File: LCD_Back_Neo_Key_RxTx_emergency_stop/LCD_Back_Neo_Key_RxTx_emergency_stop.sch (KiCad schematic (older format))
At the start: 4 parts, among them J3 Conn_01x08_Male_KeyPad, U1 DC-DC_Stepdown-Zimprich

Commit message: update
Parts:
- A1: symbol MCU_Module:Arduino_Nano_v3.x -> LCD_Back_Neo_Key_RxTx_emergency_stop-rescue:Arduino_Nano_v3.x-MCU_Module
- J3: symbol Connector:Conn_01x08_Male -> LCD_Back_Neo_Key_RxTx_emergency_stop-rescue:Conn_01x08_Male-Connector
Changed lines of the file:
@@
 $EndDescr
 $Comp
-L MCU_Module:Arduino_Nano_v3.x A1
+L LCD_Back_Neo_Key_RxTx_emergency_stop-rescue:Arduino_Nano_v3.x-MCU_Module A1
 U 1 1 5CDFD485
 P 5400 4650
@@
 Ardu_A2
 $Comp
-L Connector:Conn_01x08_Male J3
+L LCD_Back_Neo_Key_RxTx_emergency_stop-rescue:Conn_01x08_Male-Connector J3
 U 1 1 5CE28136
 P 1400 6500

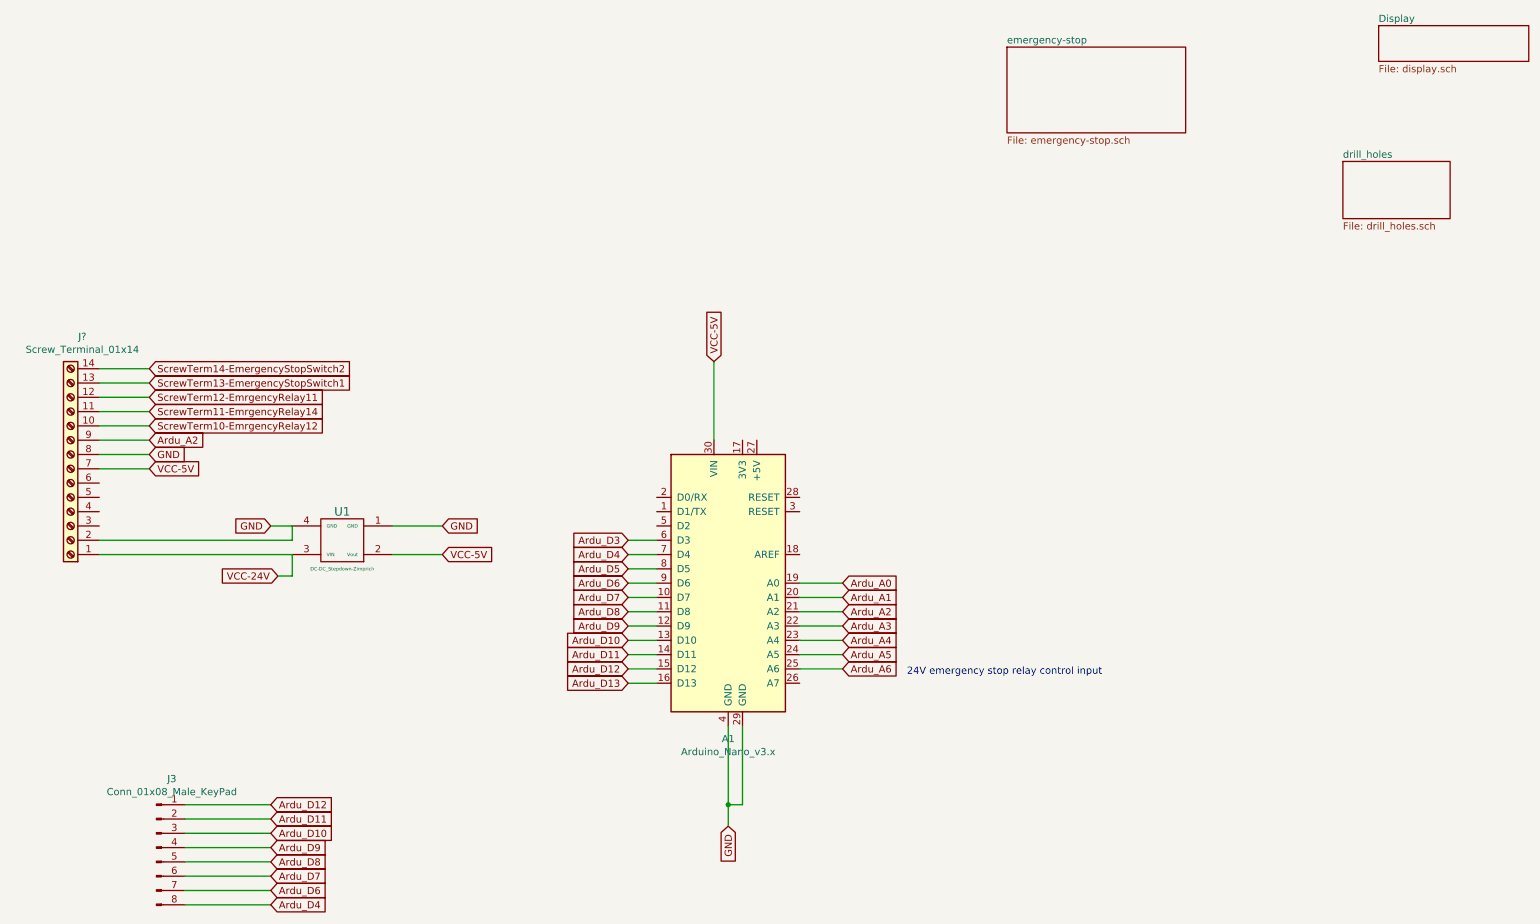
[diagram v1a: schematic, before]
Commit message: place screwterminal on PCB
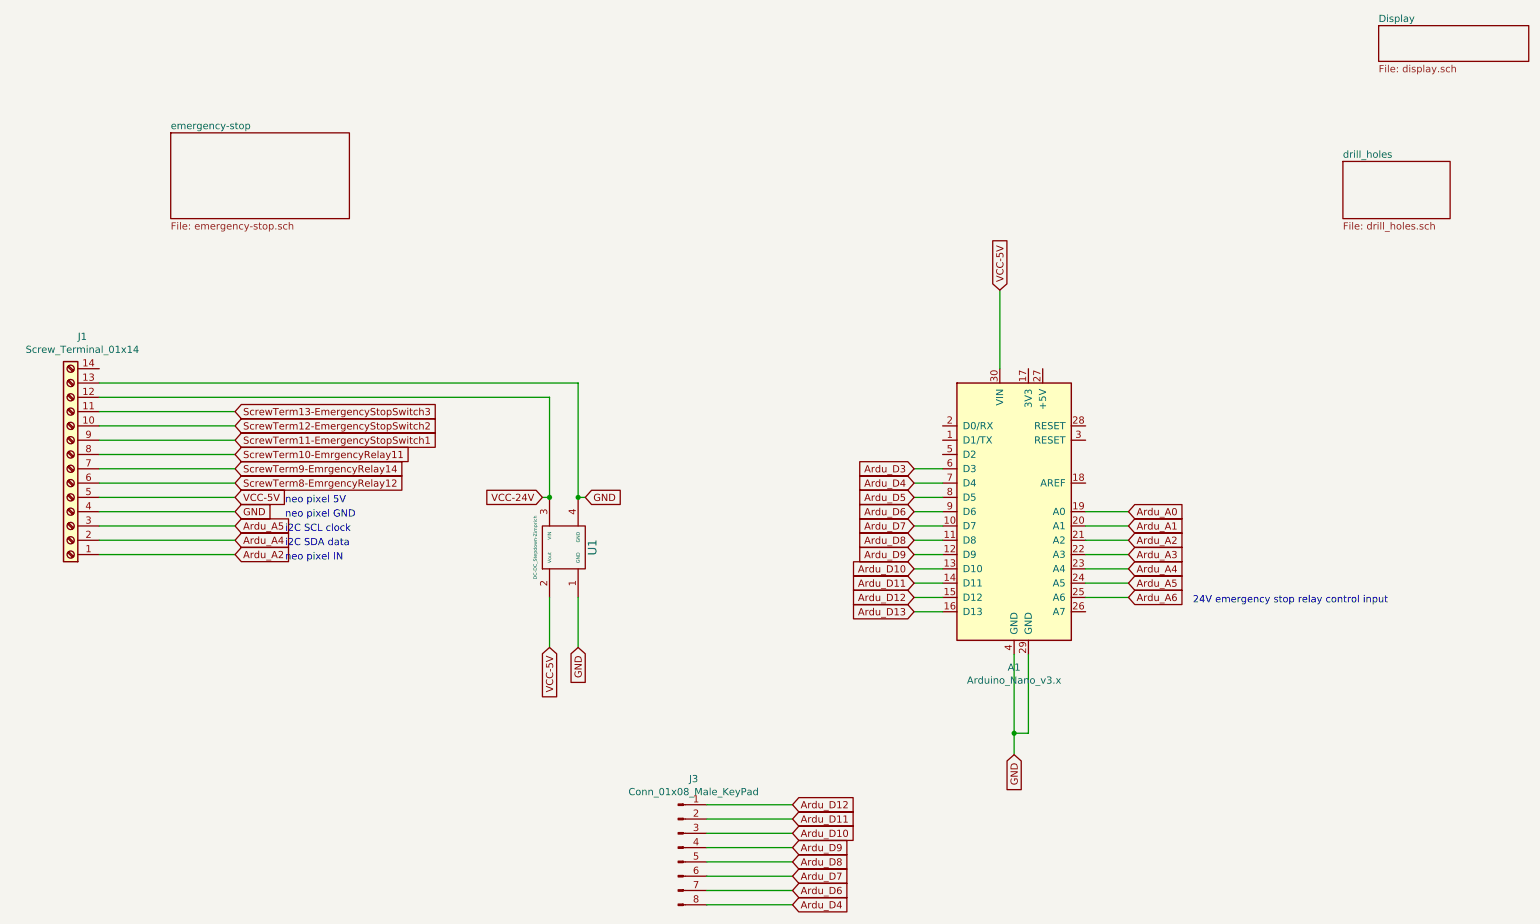
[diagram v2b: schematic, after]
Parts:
- J1: renamed from J?; footprint (none) -> Connector_Phoenix_MSTB:PhoenixContact_MSTBVA_2,5_14-G_1x14_P5.00mm_Vertical
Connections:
- net ScrewTerm12-EmrgencyRelay11 is gone; now on net VCC-24V: J1.12 (Pin_12)
- net ScrewTerm13-EmergencyStopSwitch1 is gone; now on net GND: J1.13 (Pin_13)
- net Ardu_A2: now also J1.1 (Pin_1); no longer J1.9 (Pin_9)
- net Ardu_A4: now also J1.2 (Pin_2)
- net Ardu_A5: now also J1.3 (Pin_3)
- net GND: now also J1.4 (Pin_4); no longer J1.2 (Pin_2), J1.8 (Pin_8)
- net VCC-24V: no longer J1.1 (Pin_1)
- net VCC-5V: now also J1.5 (Pin_5); no longer J1.7 (Pin_7)
- net ScrewTerm8-EmrgencyRelay12: now reaches J1.6 (Pin_6)
- net ScrewTerm10-EmrgencyRelay12 renamed ScrewTerm12-EmergencyStopSwitch2
- net ScrewTerm11-EmrgencyRelay14 renamed ScrewTerm13-EmergencyStopSwitch3
- net ScrewTerm14-EmergencyStopSwitch2: no longer names the net of J1.14 (Pin_14)
- new net ScrewTerm10-EmrgencyRelay11: J1.8 (Pin_8)
- new net ScrewTerm11-EmergencyStopSwitch1: J1.9 (Pin_9)
- new net ScrewTerm9-EmrgencyRelay14: J1.7 (Pin_7)
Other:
- note added: "i2C SCL clock"
- note added: "i2C SDA data"
- note added: "neo pixel 5V"
- note added: "neo pixel GND"
- note added: "neo pixel IN"
- moved on the sheet: A1, J3, U1
